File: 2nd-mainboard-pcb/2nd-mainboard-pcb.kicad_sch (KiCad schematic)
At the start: 30 parts, among them J1 PJ-082BH, U1 SQJ409EP-T1_GE3, U2 SZ1SMB5927BT3G, U3 TPS56837HRPAR, U4 TPS565208

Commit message: noch mehr bauteile ausgetauscht
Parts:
- R2: footprint Resistor_SMD:R_0402_1005Metric -> Resistor_SMD:R_0603_1608Metric
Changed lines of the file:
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@@
 			)
 		)
-		(property "Footprint" "Resistor_SMD:R_0402_1005Metric"
+		(property "Footprint" "Resistor_SMD:R_0603_1608Metric"
 			(at 203.962 59.69 90)
 			(effects

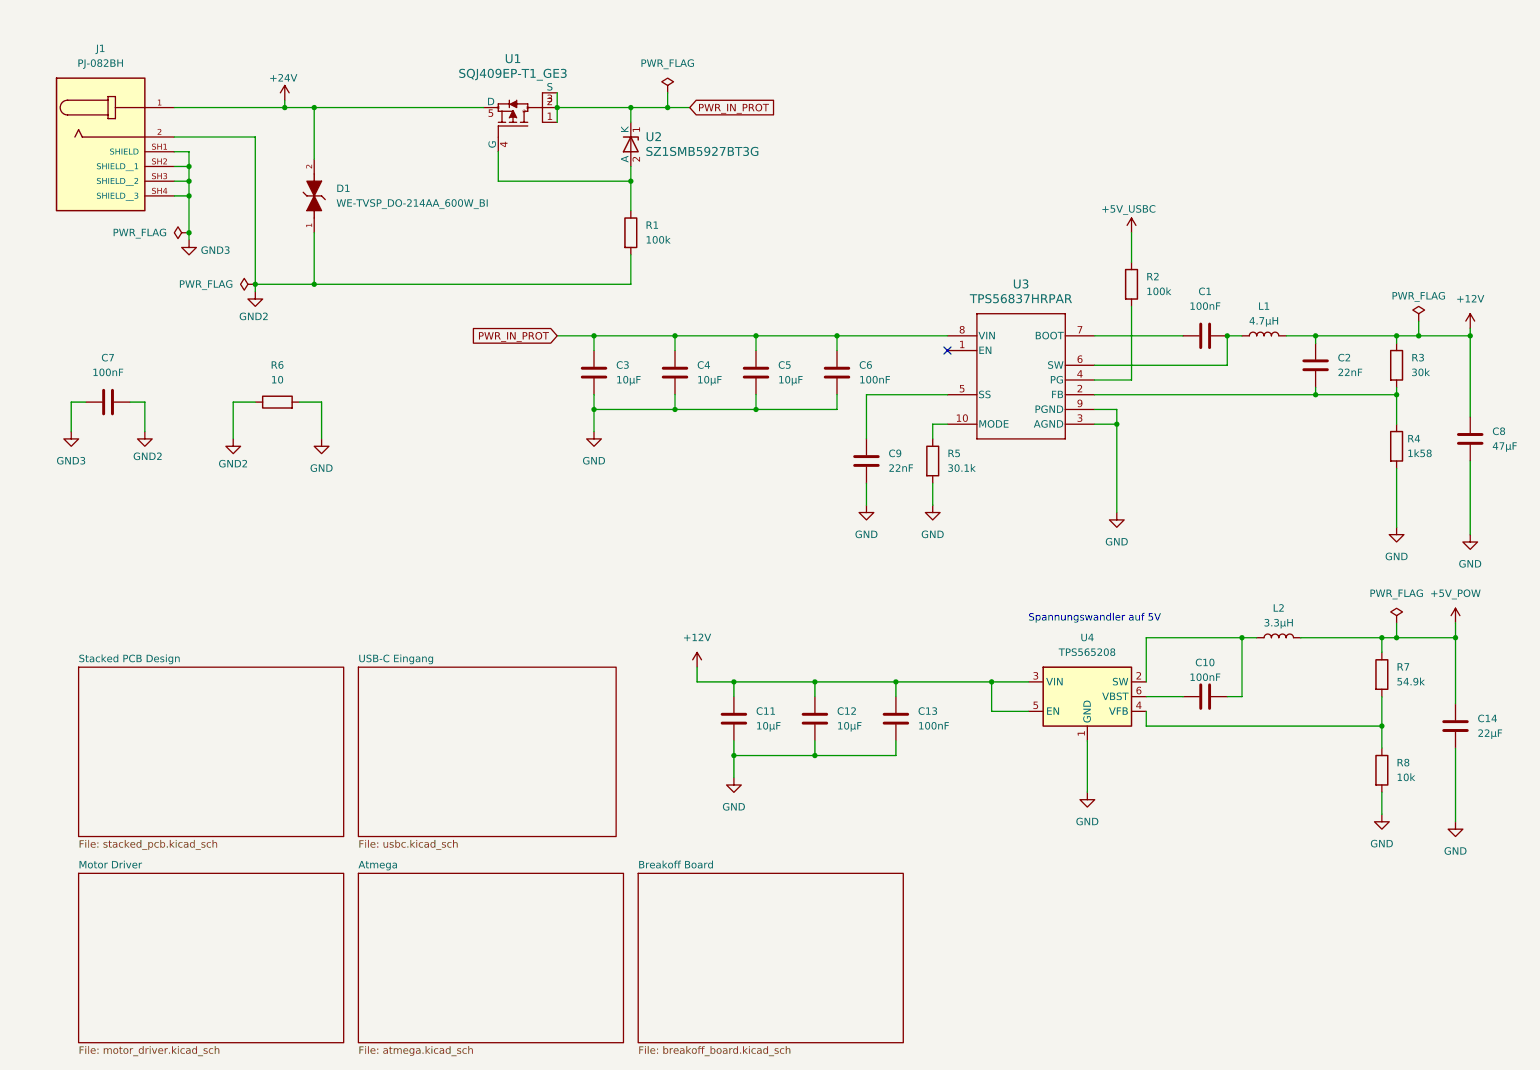
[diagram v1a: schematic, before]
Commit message: stacked pcb reworked
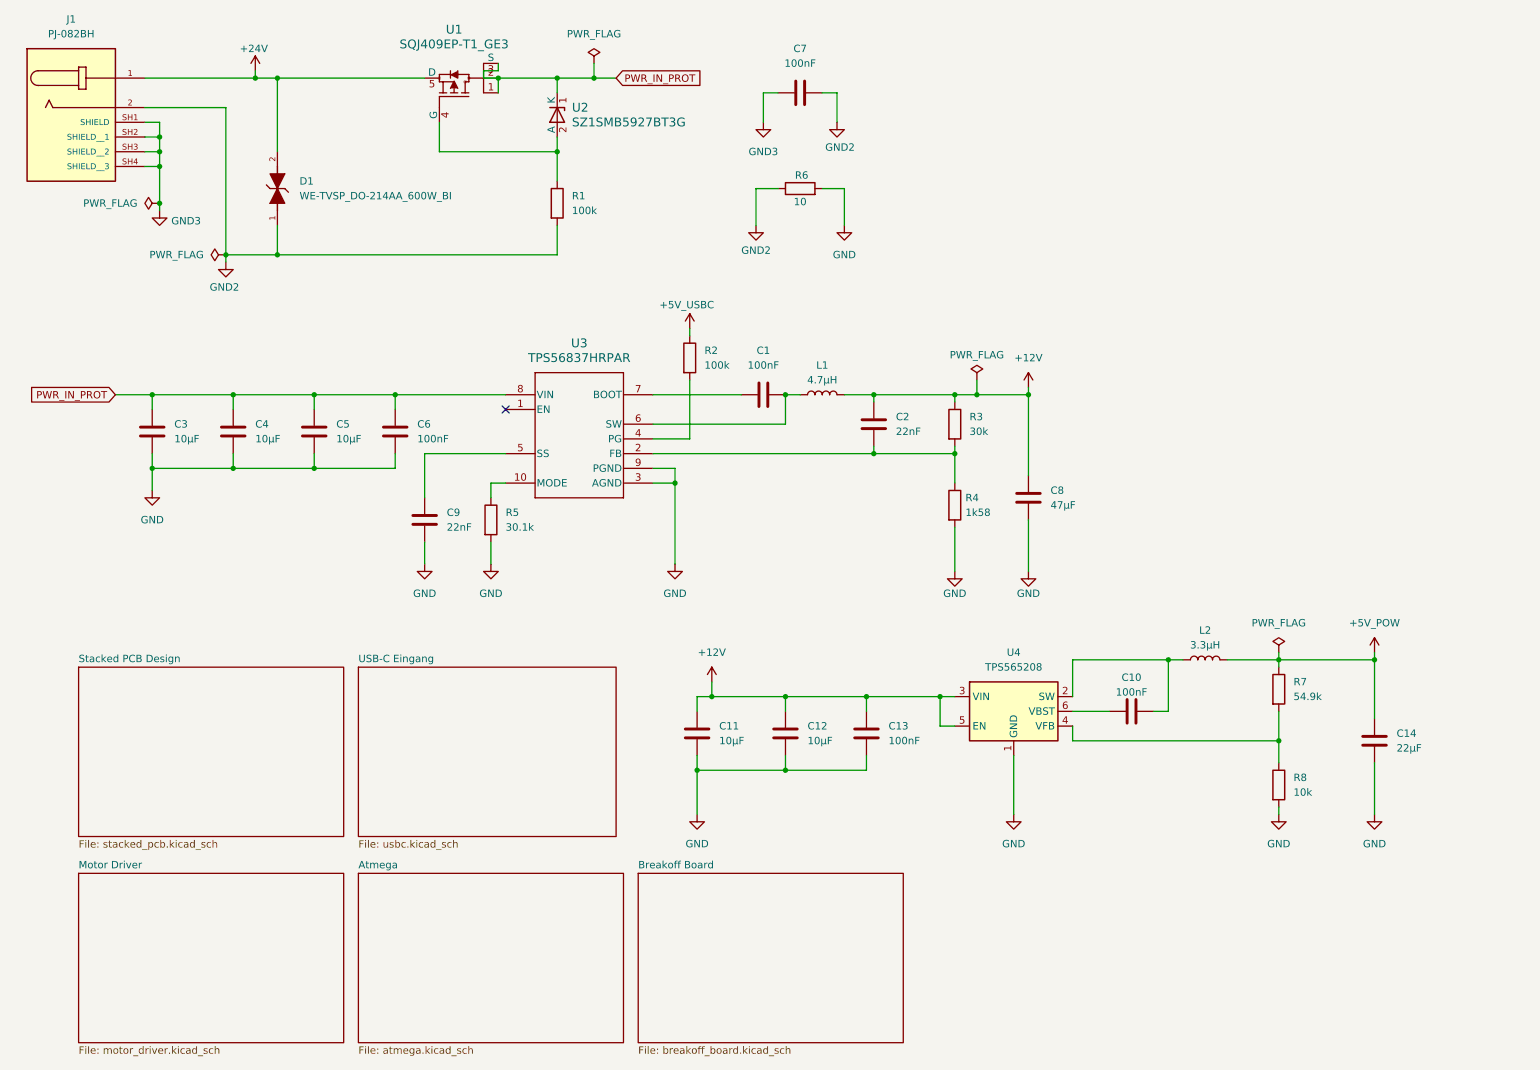
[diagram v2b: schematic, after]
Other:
- note removed: "Spannungswandler auf 5V"
- moved on the sheet: C1, C10, C11, C12, C13, C14, C2, C3, C4, C5, C6, C7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
